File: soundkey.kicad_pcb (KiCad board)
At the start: 2 copper layers, 45.9 x 20.5 mm, 38 parts, among them J1 button, J2 daughter_Pad, J3 USB_C_Receptacle_USB2.0_16P, J4 main_Pad, J5 UPDI, Q1 AO3401A, Q2 AO3401A, U1 AVR32DU28x-xSTX, U2 TP4057, U3 PAM8301, U4 TLV9001IDCK

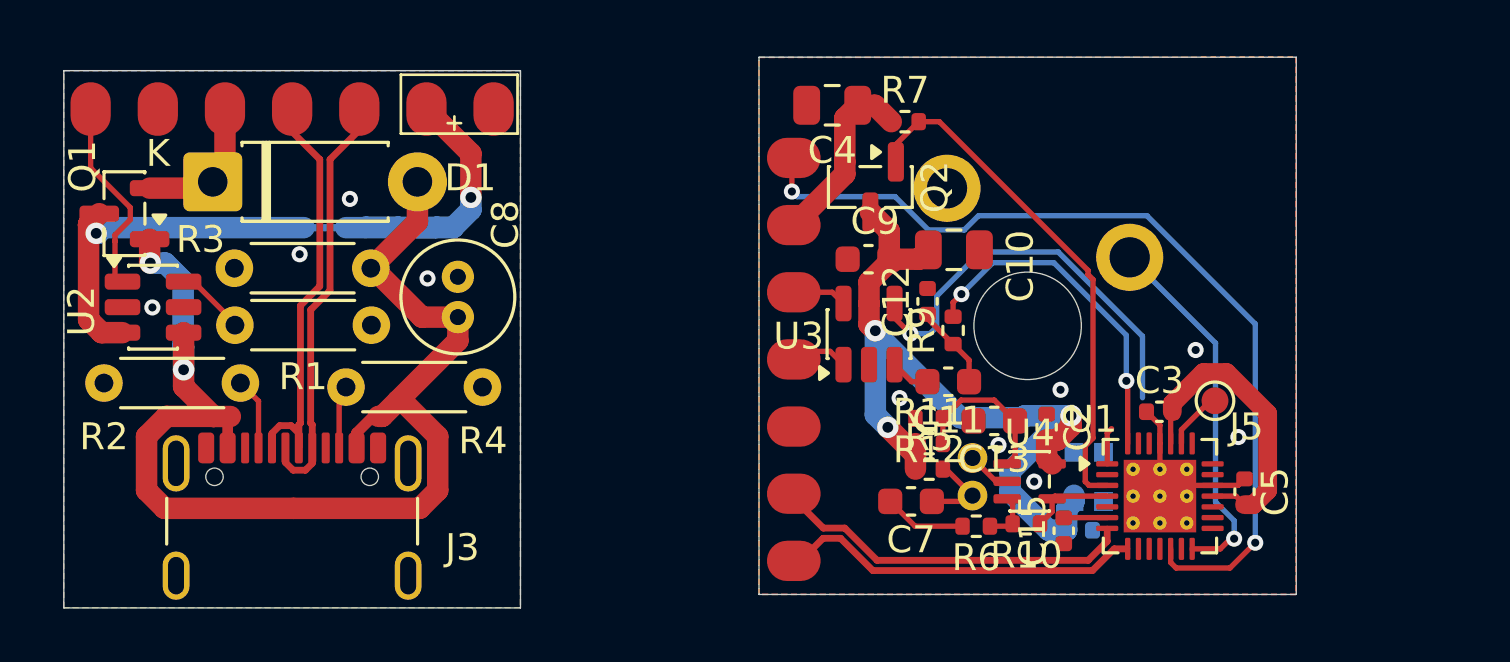
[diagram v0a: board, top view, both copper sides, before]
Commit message: 2608310153_ready for vcut
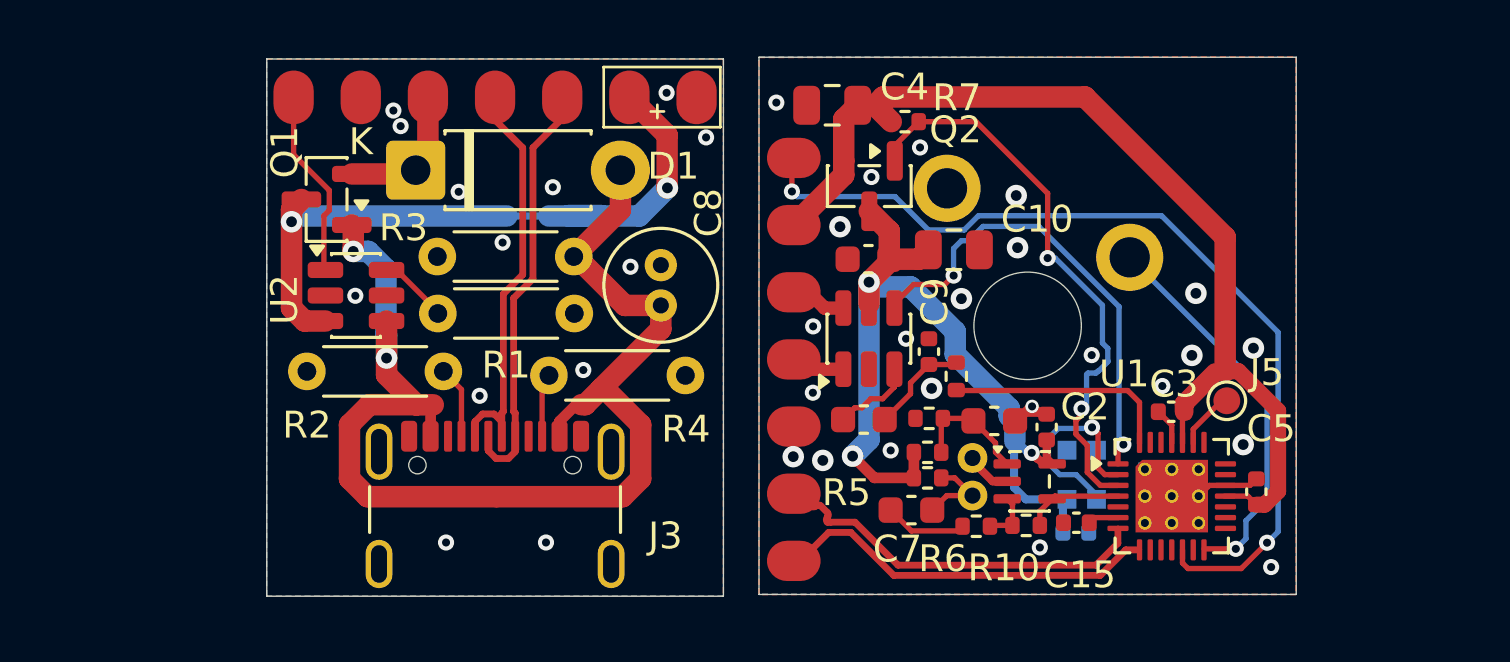
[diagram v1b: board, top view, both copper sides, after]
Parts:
- U1: footprint Package_DFN_QFN:WQFN-28-1EP_4x4mm_P0.4mm_EP2.7x2.7mm_ThermalVias -> 1_Library:VQFN-28-1EP_4x4mm_P0.4mm_EP2.7x2.7mm_ThermalVias
- moved R4 7.57 mm to (124.2, 158.8)
- moved U2 7.57 mm to (117.0, 155.9)
- moved R1 7.57 mm to (125.1, 156.5)
- moved R2 7.57 mm to (115.2, 158.7)
- moved R3 7.57 mm to (120.0, 154.4)
- moved C8 7.57 mm to (128.3, 156.2)
- moved J2 7.57 mm to (122.2, 148.5)
- moved D1 7.57 mm to (119.2, 151.2)
- moved J3 7.57 mm to (122.2, 164.8)
- moved Q1 7.54 mm to (115.9, 152.3)
- moved C11 3.44 mm to (135.9, 160.5)
- moved C12 1.87 mm to (138.3, 158.0)
- moved R9 1.71 mm to (139.3, 158.9), turned to -90 degrees
- moved C15 0.56 mm to (143.8, 164.3), turned to 0 degrees
- moved C3 0.44 mm to (147.3, 160.2)
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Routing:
- net VSYS: track 18.4 -> 38.3 mm
- net /LED: track 0.00 -> 7.94 mm, vias 0 -> 1
- net /AUDIN: track 12.8 -> 8.54 mm, vias 2 -> 0
- net /BAT+: track 28.1 -> 25.4 mm
- net /PERIPH_EN_N: track 19.4 -> 21.5 mm, vias 0 -> 2
- net Net-(U3-IN): track 1.49 -> 3.07 mm
- net Net-(U4-+): track 5.95 -> 4.59 mm
- net GND: track 8.42 -> 9.55 mm, vias 6 -> 23
- net Net-(J1-Pin_1): track 13.8 -> 14.6 mm
- net /CHG: track 33.3 -> 34.1 mm
- net Net-(C11-Pad1): track 3.15 -> 3.92 mm
- net /D-: track 13.5 -> 14.3 mm
- net /D+: track 13.6 -> 14.3 mm
- net VCC: track 32.1 -> 32.8 mm
- net /MIC: track 3.21 -> 3.71 mm
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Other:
- board size 45.9 x 20.5 mm -> 38.3 x 20.1 mm

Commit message: 2608310324_ready for produce(vcut canceled)
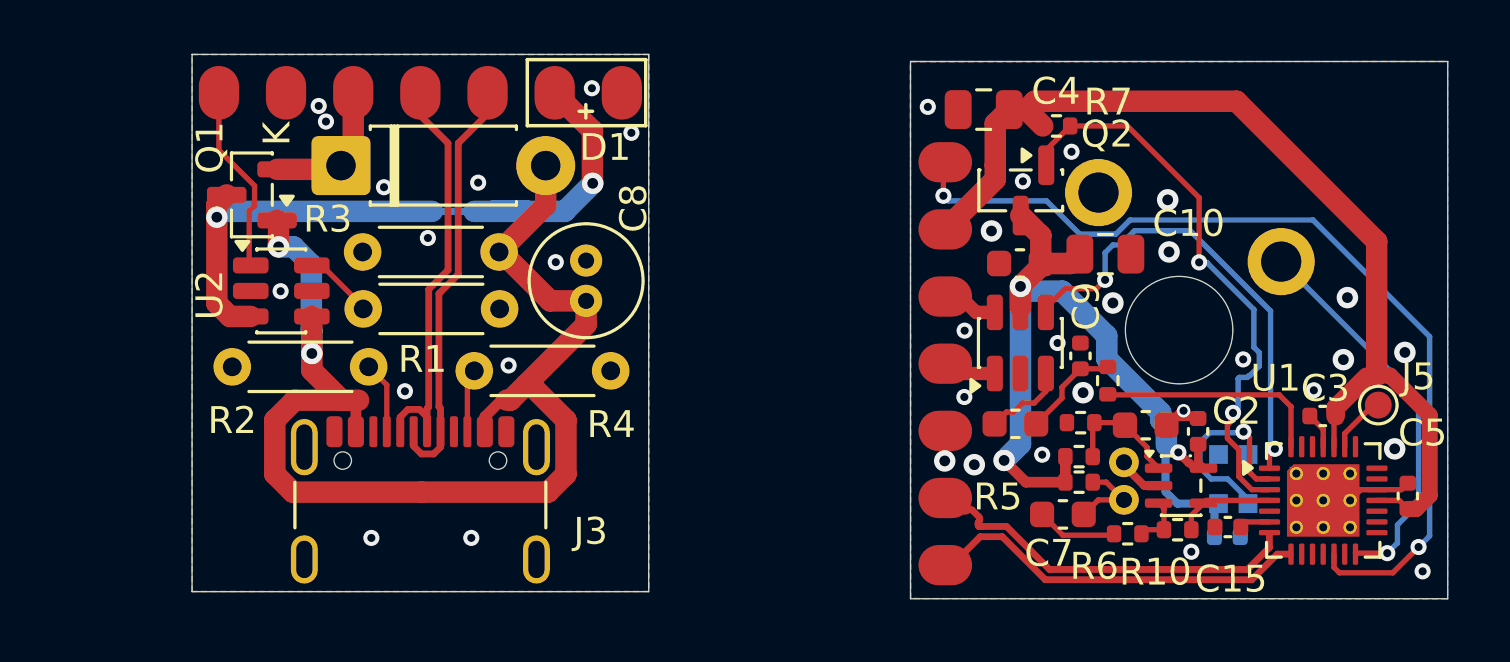
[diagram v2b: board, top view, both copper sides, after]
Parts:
- moved R6 5.65 mm to (145.7, 164.7)
- moved C14 5.64 mm to (149.4, 164.8)
- moved C5 5.64 mm to (156.2, 163.3)
- moved D2 5.64 mm to (149.7, 162.7)
- moved J4 5.64 mm to (138.9, 158.4)
- moved C10 5.64 mm to (144.9, 154.3)
- moved C11 5.64 mm to (141.5, 160.6)
- moved C12 5.64 mm to (144.0, 158.1)
- moved C13 5.64 mm to (146.4, 160.7)
- moved C15 5.64 mm to (149.5, 164.5)
- moved C2 5.64 mm to (148.3, 160.9)
- moved C3 5.64 mm to (153.0, 160.4)
- moved C4 5.64 mm to (140.4, 148.9)
- moved C7 5.64 mm to (143.3, 164.0)
- moved C9 5.64 mm to (141.7, 154.7)
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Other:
- board size 38.3 x 20.1 mm -> 46.7 x 20.3 mm
